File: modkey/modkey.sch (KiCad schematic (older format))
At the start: 12 parts, among them J1 Conn_01x04, J2 Conn_01x04, J3 Conn_01x04, J4 Conn_01x04, SW1 SW_Push, U1 ATtiny85-20SU

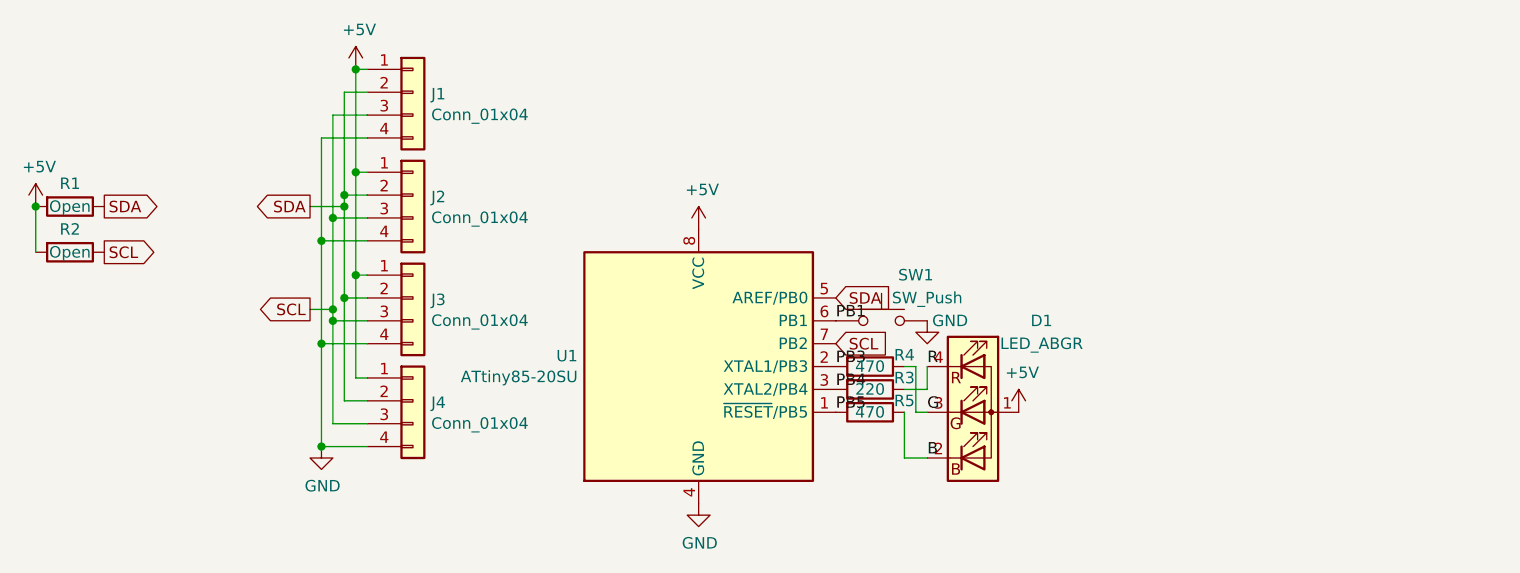
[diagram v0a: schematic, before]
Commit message: update
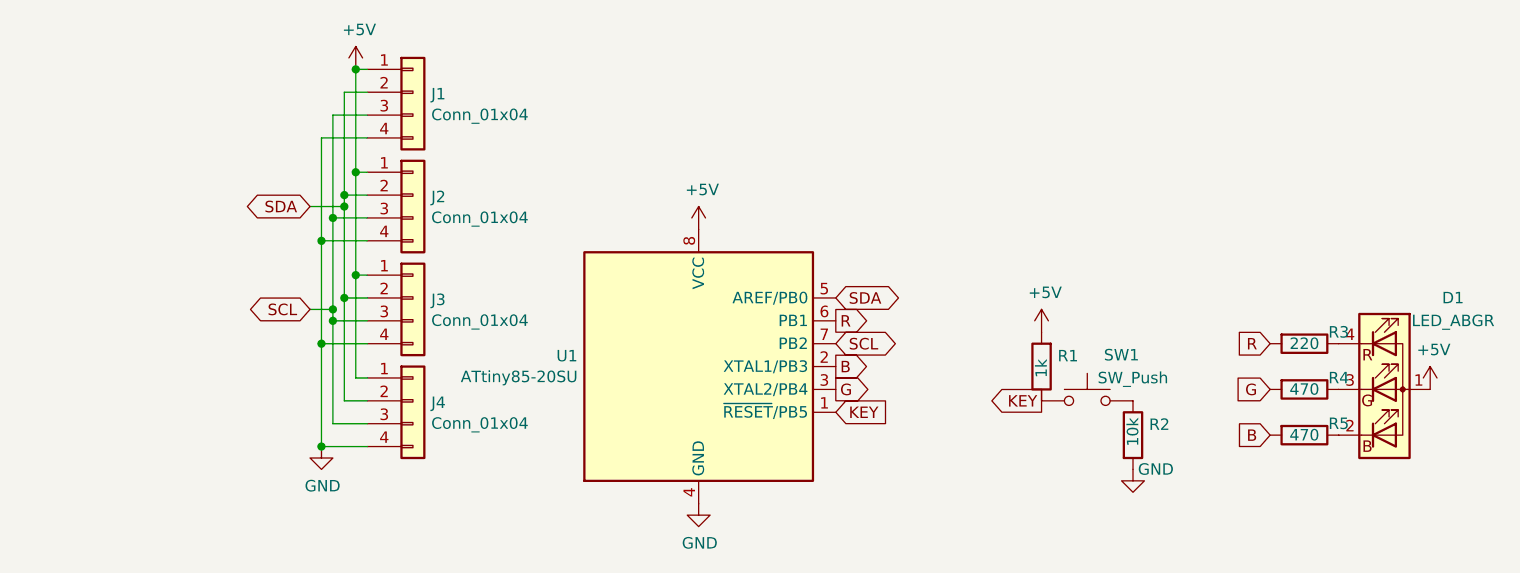
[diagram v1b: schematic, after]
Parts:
- R1: value Open -> 1k; footprint Resistor_SMD:R_0805_2012Metric_Pad1.15x1.40mm_HandSolder -> Resistor_SMD:R_0805_2012Metric_Pad1.20x1.40mm_HandSolder
- R2: value Open -> 10k; footprint Resistor_SMD:R_0805_2012Metric_Pad1.15x1.40mm_HandSolder -> Resistor_SMD:R_0805_2012Metric_Pad1.20x1.40mm_HandSolder
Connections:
- net +5V: no longer R2.2
- net B: now also R5.2, U1.2 (XTAL1/PB3); no longer D1.2 (BK), R5.1
- net G: now also R4.2, U1.3 (XTAL2/PB4); no longer D1.3 (GK), R4.1
- net GND: now also R2.2; no longer SW1.2
- net R: now also R3.2, U1.6 (PB1); no longer D1.4 (RK), R3.1
- net SCL: no longer R2.1
- net SDA: no longer R1.1
- net PB1 renamed KEY
- net KEY: now also R1.1, U1.1 (~RESET~/PB5); no longer U1.6 (PB1)
- removed net PB3: R4.2, U1.2 (XTAL1/PB3)
- removed net PB4: R3.2, U1.3 (XTAL2/PB4)
- removed net PB5: R5.2, U1.1 (~RESET~/PB5)
- new net: D1.2 (BK), R5.1
- new net: D1.3 (GK), R4.1
- new net: D1.4 (RK), R3.1
- new net: R2.1, SW1.2
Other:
- moved on the sheet: D1, R3, R4, R5, SW1
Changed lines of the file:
@@
 	1    0    0    -1
 $EndComp
-Text GLabel 5350 1850 2    50   Input ~ 0
+Text GLabel 5350 1850 2    50   BiDi ~ 0
 SDA
-Text GLabel 5350 2050 2    50   Input ~ 0
+Text GLabel 5350 2050 2    50   BiDi ~ 0
 SCL
 $Comp
@@
 L Device:LED_ABGR D1
 U 1 1 5E3911C3
-P 5950 2350
-F 0 "D1" H 6250 2750 50  0000 C CNN
-F 1 "LED_ABGR" H 6250 2650 50  0000 C CNN
-F 2 "LED_SMD:LED_Cree-PLCC4_2x2mm_CW" H 5950 2350 50  0001 C CNN
-F 3 "~" H 5950 2350 50  0001 C CNN
-	1    5950 2350
+P 7750 2250
+F 0 "D1" H 8050 2650 50  0000 C CNN
+F 1 "LED_ABGR" H 8050 2550 50  0000 C CNN
+F 2 "LED_SMD:LED_Cree-PLCC4_2x2mm_CW" H 7750 2250 50  0001 C CNN
+F 3 "~" H 7750 2250 50  0001 C CNN
+	1    7750 2250
 	1    0    0    -1
 $EndComp
@@
 L Device:R R3
 U 1 1 5E39414A
-P 5500 2250
-F 0 "R3" V 5450 2400 50  0000 C CNN
-F 1 "220" V 5500 2250 50  0000 C CNN
-F 2 "Resistor_SMD:R_0805_2012Metric_Pad1.15x1.40mm_HandSolder" V 5430 2250 50  0001 C CNN
-F 3 "~" H 5500 2250 50  0001 C CNN
-	1    5500 2250
+P 7400 2050
+F 0 "R3" V 7350 2200 50  0000 C CNN
+F 1 "220" V 7400 2050 50  0000 C CNN
+F 2 "Resistor_SMD:R_0805_2012Metric_Pad1.15x1.40mm_HandSolder" V 7330 2050 50  0001 C CNN
+F 3 "~" H 7400 2050 50  0001 C CNN
+	1    7400 2050
 	0    1    1    0
 $EndComp
@@
 L Device:R R5
 U 1 1 5E395A5F
-P 5500 2350
-F 0 "R5" V 5450 2500 50  0000 C CNN
-F 1 "470" V 5500 2350 50  0000 C CNN
-F 2 "Resistor_SMD:R_0805_2012Metric_Pad1.15x1.40mm_HandSolder" V 5430 2350 50  0001 C CNN
-F 3 "~" H 5500 2350 50  0001 C CNN
-	1    5500 2350
+P 7400 2450
+F 0 "R5" V 7350 2600 50  0000 C CNN
+F 1 "470" V 7400 2450 50  0000 C CNN
+F 2 "Resistor_SMD:R_0805_2012Metric_Pad1.15x1.40mm_HandSolder" V 7330 2450 50  0001 C CNN
+F 3 "~" H 7400 2450 50  0001 C CNN
+	1    7400 2450
 	0    1    1    0
 $EndComp
-Wire Wire Line
-	5650 2350 5650 2550
 $Comp
 L power:+5V #PWR0103
 U 1 1 5E3962CE
-P 6150 2350
-F 0 "#PWR0103" H 6150 2200 50  0001 C CNN
-F 1 "+5V" H 6165 2523 50  0000 C CNN
-F 2 "" H 6150 2350 50  0001 C CNN
-F 3 "" H 6150 2350 50  0001 C CNN
-	1    6150 2350
+P 7950 2250
+F 0 "#PWR0103" H 7950 2100 50  0001 C CNN
+F 1 "+5V" H 7965 2423 50  0000 C CNN
+F 2 "" H 7950 2250 50  0001 C CNN
+F 3 "" H 7950 2250 50  0001 C CNN
+	1    7950 2250
 	1    0    0    -1
 $EndComp
@@
 L Switch:SW_Push SW1
 U 1 1 5E396E33
-P 5550 1950
-F 0 "SW1" H 5700 2150 50  0000 C CNN
-F 1 "SW_Push" H 5750 2050 50  0000 C CNN
-F 2 "gHeavyIndustries:MX-Alps-Choc-X-1U-NoLED" H 5550 2150 50  0001 C CNN
-F 3 "~" H 5550 2150 50  0001 C CNN
-	1    5550 1950
+P 6450 2300
+F 0 "SW1" H 6600 2500 50  0000 C CNN
+F 1 "SW_Push" H 6650 2400 50  0000 C CNN
+F 2 "gHeavyIndustries:MX-Alps-Choc-X-1U-NoLED" H 6450 2500 50  0001 C CNN
+F 3 "~" H 6450 2500 50  0001 C CNN
+	1    6450 2300
 	1    0    0    -1
 $EndComp
@@
 L power:GND #PWR0104
 U 1 1 5E3976C0
-P 5750 1950
-F 0 "#PWR0104" H 5750 1700 50  0001 C CNN
-F 1 "GND" H 5850 1950 50  0000 C CNN
-F 2 "" H 5750 1950 50  0001 C CNN
-F 3 "" H 5750 1950 50  0001 C CNN
-	1    5750 1950
+P 6650 2600
+F 0 "#PWR0104" H 6650 2350 50  0001 C CNN
+F 1 "GND" H 6750 2600 50  0000 C CNN
+F 2 "" H 6650 2600 50  0001 C CNN
+F 3 "" H 6650 2600 50  0001 C CNN
+	1    6650 2600
 	1    0    0    -1
 $EndComp
@@
 Wire Wire Line
 	3100 2500 3300 2500
-Text GLabel 3050 1450 0    50   Output ~ 0
+Text GLabel 3050 1450 0    50   BiDi ~ 0
 SDA
-Text GLabel 3050 1900 0    50   Output ~ 0
+Text GLabel 3050 1900 0    50   BiDi ~ 0
 SCL
 Wire Wire Line
@@
 	3150 1900 3150 1950
 $Comp
-L Device:R R1
-U 1 1 5E3A1459
-P 2000 1450
-F 0 "R1" V 1900 1450 50  0000 C CNN
-F 1 "Open" V 2000 1450 50  0000 C CNN
-F 2 "Resistor_SMD:R_0805_2012Metric_Pad1.15x1.40mm_HandSolder" V 1930 1450 50  0001 C CNN
-F 3 "~" H 2000 1450 50  0001 C CNN
-	1    2000 1450
-	0    1    1    0
-$EndComp
-$Comp
-L Device:R R2
-U 1 1 5E3A1738
-P 2000 1650
-F 0 "R2" V 1900 1650 50  0000 C CNN
-F 1 "Open" V 2000 1650 50  0000 C CNN
-F 2 "Resistor_SMD:R_0805_2012Metric_Pad1.15x1.40mm_HandSolder" V 1930 1650 50  0001 C CNN
-F 3 "~" H 2000 1650 50  0001 C CNN
-	1    2000 1650
-	0    1    1    0
-$EndComp
-Text GLabel 2150 1450 2    50   Output ~ 0
-SDA
-Text GLabel 2150 1650 2    50   Output ~ 0
-SCL
-$Comp
-L power:+5V #PWR0107
-U 1 1 5E3A2531
-P 1850 1450
-F 0 "#PWR0107" H 1850 1300 50  0001 C CNN
-F 1 "+5V" H 1865 1623 50  0000 C CNN
-F 2 "" H 1850 1450 50  0001 C CNN
-F 3 "" H 1850 1450 50  0001 C CNN
-	1    1850 1450
-	1    0    0    -1
-$EndComp
-Wire Wire Line
-	1850 1450 1850 1650
-Connection ~ 1850 1450
-Text Label 5750 2150 0    50   ~ 0
-R
-Text Label 5750 2550 0    50   ~ 0
-B
-Text Label 5350 2150 0    50   ~ 0
-PB3
-Text Label 5350 2250 0    50   ~ 0
-PB4
-Text Label 5350 2350 0    50   ~ 0
-PB5
-Text Label 5350 1950 0    50   ~ 0
-PB1
-$Comp
 L Device:R R4
 U 1 1 5E395817
-P 5500 2150
-F 0 "R4" V 5450 2300 50  0000 C CNN
-F 1 "470" V 5500 2150 50  0000 C CNN
-F 2 "Resistor_SMD:R_0805_2012Metric_Pad1.15x1.40mm_HandSolder" V 5430 2150 50  0001 C CNN
-F 3 "~" H 5500 2150 50  0001 C CNN
-	1    5500 2150
+P 7400 2250
+F 0 "R4" V 7350 2400 50  0000 C CNN
+F 1 "470" V 7400 2250 50  0000 C CNN
+F 2 "Resistor_SMD:R_0805_2012Metric_Pad1.15x1.40mm_HandSolder" V 7330 2250 50  0001 C CNN
+F 3 "~" H 7400 2250 50  0001 C CNN
+	1    7400 2250
 	0    1    1    0
 $EndComp
-Text Label 5750 2350 0    50   ~ 0
+$Comp
+L Device:R R1
+U 1 1 60BEC7C9
+P 6250 2150
+F 0 "R1" H 6180 2104 50  0000 R CNN
+F 1 "1k" V 6250 2200 50  0000 R CNN
+F 2 "Resistor_SMD:R_0805_2012Metric_Pad1.20x1.40mm_HandSolder" V 6180 2150 50  0001 C CNN
+F 3 "~" H 6250 2150 50  0001 C CNN
+	1    6250 2150
+	-1   0    0    1
+$EndComp
+$Comp
+L Device:R R2
+U 1 1 60BECCA7
+P 6650 2450
+F 0 "R2" H 6720 2496 50  0000 L CNN
+F 1 "10k" V 6650 2400 50  0000 L CNN
+F 2 "Resistor_SMD:R_0805_2012Metric_Pad1.20x1.40mm_HandSolder" V 6580 2450 50  0001 C CNN
+F 3 "~" H 6650 2450 50  0001 C CNN
+	1    6650 2450
+	1    0    0    -1
+$EndComp
+Text GLabel 7250 2050 0    50   Input ~ 0
+R
+Text GLabel 7250 2250 0    50   Input ~ 0
 G
-Wire Wire Line
-	5650 2550 5750 2550
-Wire Wire Line
-	5750 2350 5700 2350
-Wire Wire Line
-	5700 2350 5700 2150
-Wire Wire Line
-	5700 2150 5650 2150
-Wire Wire Line
-	5750 2150 5750 2250
-Wire Wire Line
-	5750 2250 5650 2250
+Text GLabel 7250 2450 0    50   Input ~ 0
+B
+$Comp
+L power:+5V #PWR01
+U 1 1 60BFAE59
+P 6250 2000
+F 0 "#PWR01" H 6250 1850 50  0001 C CNN
+F 1 "+5V" H 6265 2173 50  0000 C CNN
+F 2 "" H 6250 2000 50  0001 C CNN
+F 3 "" H 6250 2000 50  0001 C CNN
+	1    6250 2000
+	1    0    0    -1
+$EndComp
+Text GLabel 5350 1950 2    50   Output ~ 0
+R
+Text GLabel 5350 2250 2    50   Output ~ 0
+G
+Text GLabel 5350 2150 2    50   Output ~ 0
+B
+Text GLabel 6250 2300 0    50   Output ~ 0
+KEY
+Text GLabel 5350 2350 2    50   Input ~ 0
+KEY
 $EndSCHEMATC
